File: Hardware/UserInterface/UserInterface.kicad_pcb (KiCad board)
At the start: 4 copper layers, 66.8 x 26 mm, 68 parts, among them J101 conn_turnSignal, J102 conn_OLED, J103 conn_joystick, J201 TagConnect_SWD, J202 USB_C_Receptacle_USB2.0_16P, J301 RJ9, J302 RJ9, SW201 SW_Push, SW202 SW_Push, U201 W25Q64JVXGIQ, U202 RP2040, U301 MCP2551-I-SN, U302 MCP2515-xST, U303 AP63203WU, U304 AP63205WU, Y201 12M, Y301 8M

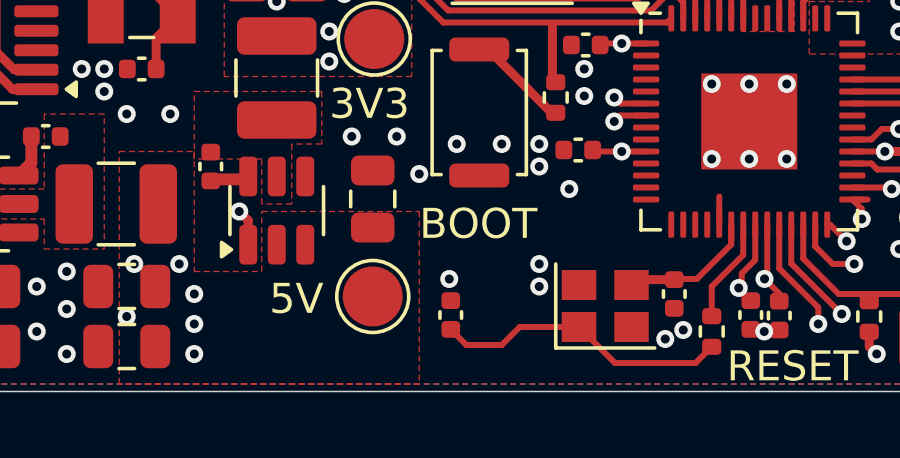
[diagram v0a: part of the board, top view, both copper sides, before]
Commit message: Add software files
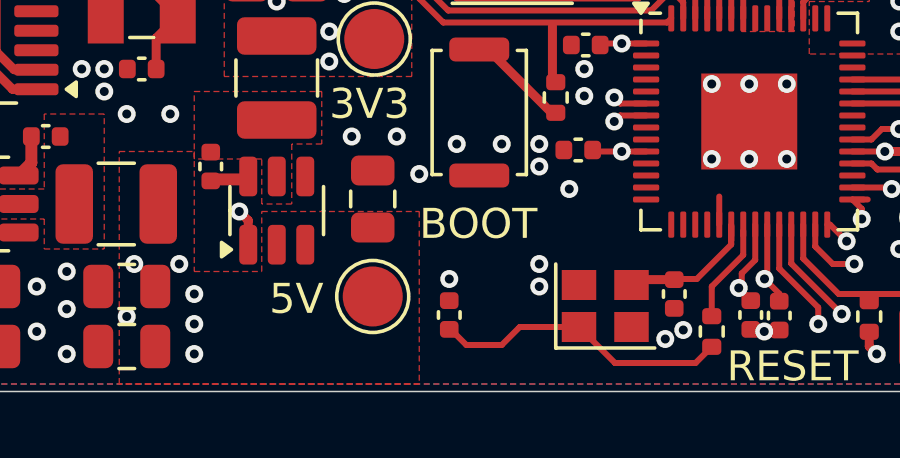
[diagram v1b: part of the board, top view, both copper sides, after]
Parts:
- moved C215 0.05 mm to (130.5, 52.7)
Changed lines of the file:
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@@
 	(footprint "Capacitor_SMD:C_0402_1005Metric"
 		(layer "F.Cu")
-		(at 130.55 52.7 -90)
+		(at 130.5 52.7 -90)
 		(descr "Capacitor SMD 0402 (1005 Metric), square (rectangular) end terminal, IPC_7351 nominal, (Body size source: IPC-SM-782 page 76, https://www.pcb-3d.com/wordpress/wp-content/uploads/ipc-sm-782a_amendment_1_and_2.pdf), generated with kicad-footprint-generator")
 		(tags "capacitor")
